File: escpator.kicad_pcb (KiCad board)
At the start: 4 copper layers, 45.7 x 15 mm, 36 parts, among them J1 Conn_01x04_Pin, J2 Conn_02x05_Odd_Even, J3 Conn_01x05, U1 STM32F103CBTx, U3 SRV05-4, U4 MCP1700x-330xxTT, X1 8MHz(12pF)

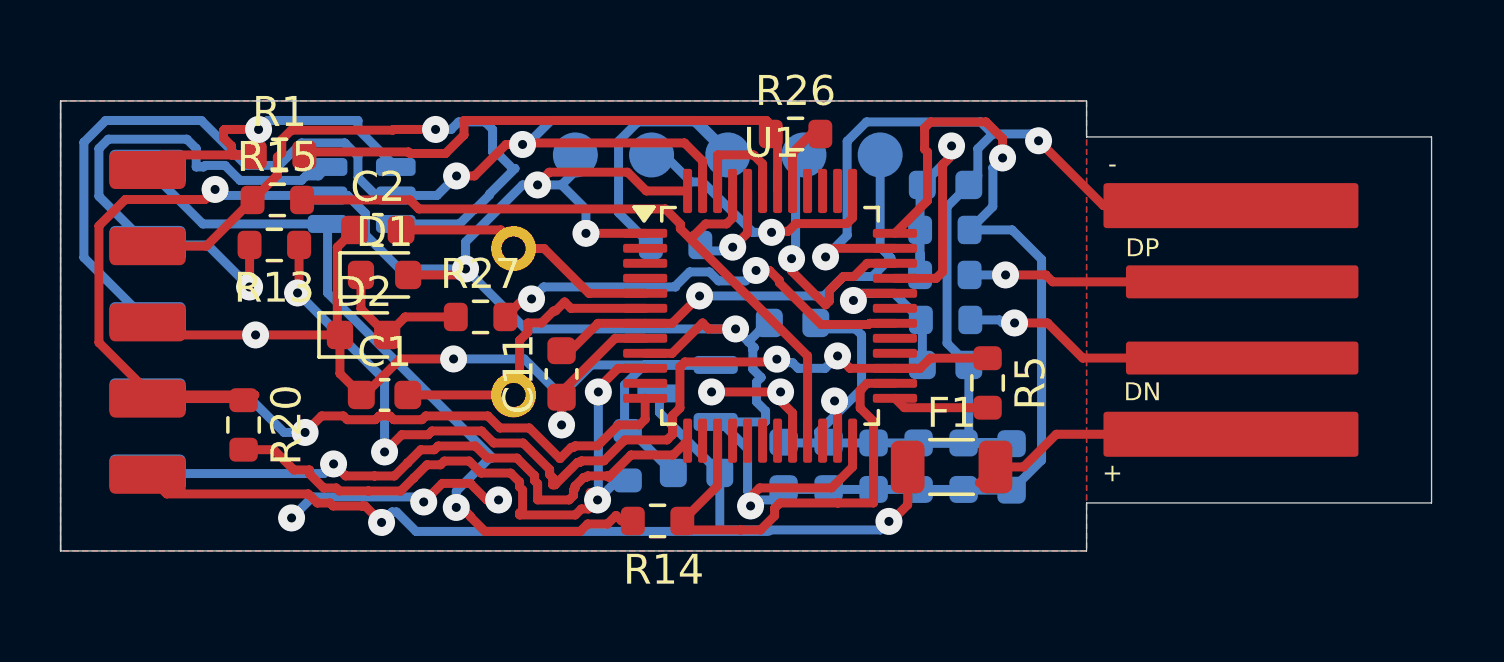
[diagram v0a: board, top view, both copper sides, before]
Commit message: second
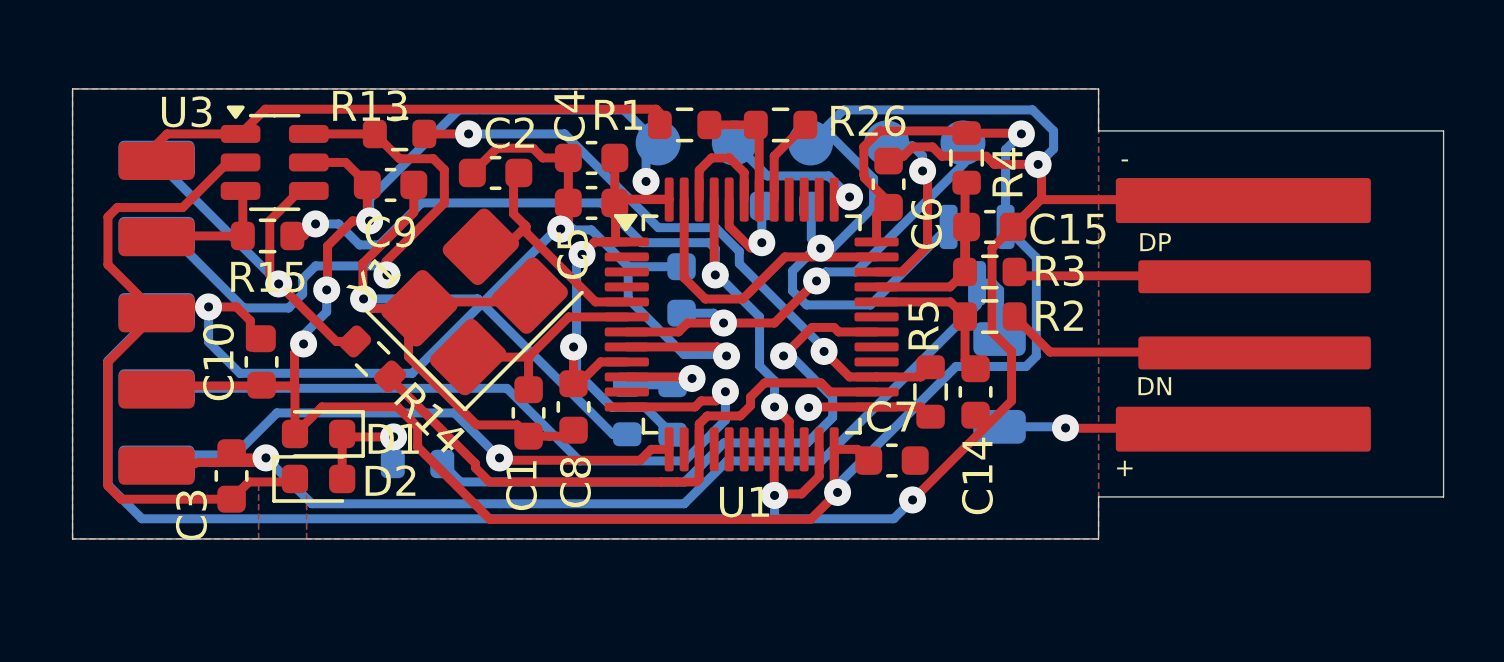
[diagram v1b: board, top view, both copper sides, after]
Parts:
- removed X1: 8MHz(12pF), Crystal:Crystal_HC49-U_Vertical
- added Y1: Crystal_GND24, Crystal:Crystal_SMD_3225-4Pin_3.2x2.5mm_HandSoldering, F.Cu at (116.5, 36.9)
- C10, C14, C15, C3, C4, C5, C6, C7, C8, C9, R2, R3, R4, U3: moved to F.Cu
- C11, F1, R20, R27: moved to B.Cu
- moved C9 21.3 mm to (113.7, 33.0), turned to 0 degrees
- moved C10 17.7 mm to (109.4, 38.9), turned to 90 degrees
- moved C4 17.4 mm to (120.4, 32.1), turned to 180 degrees
- moved C3 15.5 mm to (108.4, 42.7), turned to -90 degrees
- moved R20 14.3 mm to (123.1, 40.5), turned to 90 degrees
- moved R1 13.5 mm to (123.5, 31.0)
- moved C5 12.9 mm to (120.4, 33.6), turned to 180 degrees
- moved R14 10.9 mm to (113.1, 38.8), turned to 135 degrees
- moved U4 10.7 mm to (133.2, 35.3), turned to -90 degrees
- moved C6 10.0 mm to (130.3, 33.0)
- moved C8 8.72 mm to (119.8, 40.4), turned to -90 degrees
- moved D1 5.74 mm to (111.3, 41.3), turned to 180 degrees
- moved R13 5.58 mm to (114.0, 31.3)
- moved R27 5.33 mm to (114.6, 42.3)
- moved D2 5.03 mm to (111.3, 42.8)
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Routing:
- net Earth: track 150.7 -> 195.2 mm, vias 13 -> 8
- net /AIN1: track 21.7 -> 4.45 mm, vias 2 -> 1
- net Net-(J2-Pin_3): track 20.5 -> 5.41 mm, vias 1 -> 0
- net /T_NRST: track 18.7 -> 3.91 mm
- net /T_JTMS: track 33.1 -> 20.7 mm, vias 4 -> 2
- net Net-(J2-Pin_2): track 25.6 -> 14.1 mm
- net /STLINK_TX: track 19.3 -> 26.6 mm
- net /LED_STLINK: track 14.7 -> 20.6 mm, vias 2 -> 1
- net Net-(J2-Pin_1): track 12.2 -> 17.9 mm, vias 1 -> 0
- net /T_JTCK: track 15.4 -> 20.5 mm
- net Net-(J1-Pin_1): track 12.8 -> 8.13 mm, vias 0 -> 1
- net /USB_P: track 11.5 -> 7.57 mm, vias 1 -> 0
- net +3V3: track 103.4 -> 99.5 mm, vias 7 -> 8
- net /OSC_OUT: track 10.8 -> 6.93 mm
- net /SWCLK: track 8.73 -> 5.13 mm
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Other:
- outline, holes or cut-outs redrawn
